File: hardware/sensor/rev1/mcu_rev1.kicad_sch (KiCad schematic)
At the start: 14 parts, among them IC1 STM8L051F3P6, J1 22-28-4044, J2 M20-9770342

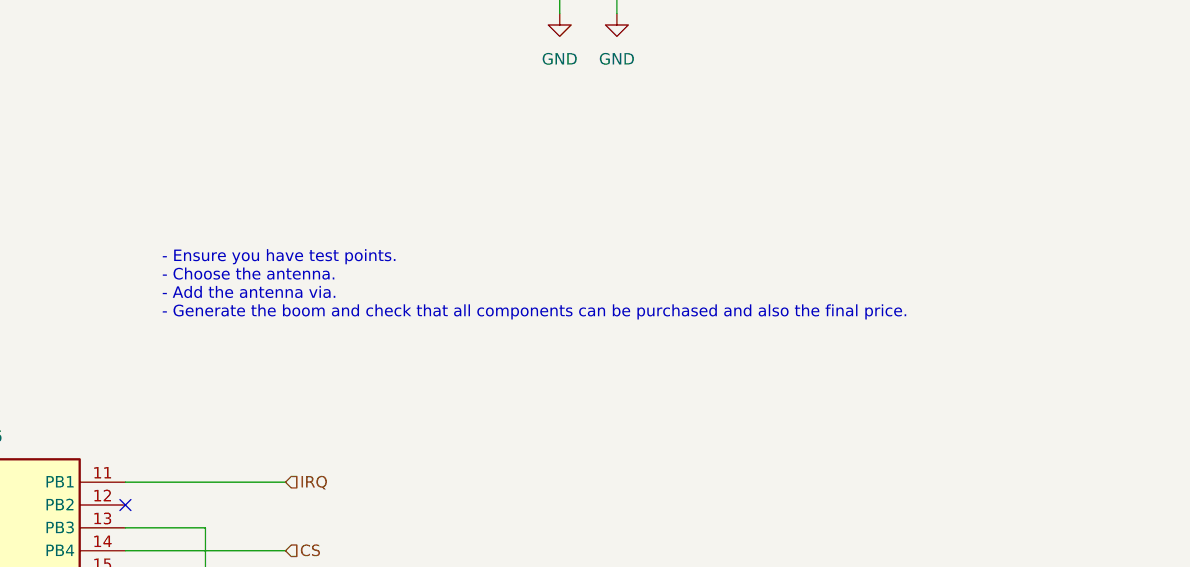
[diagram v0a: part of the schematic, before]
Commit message: EG-49 Adjust antenna place in PCB.
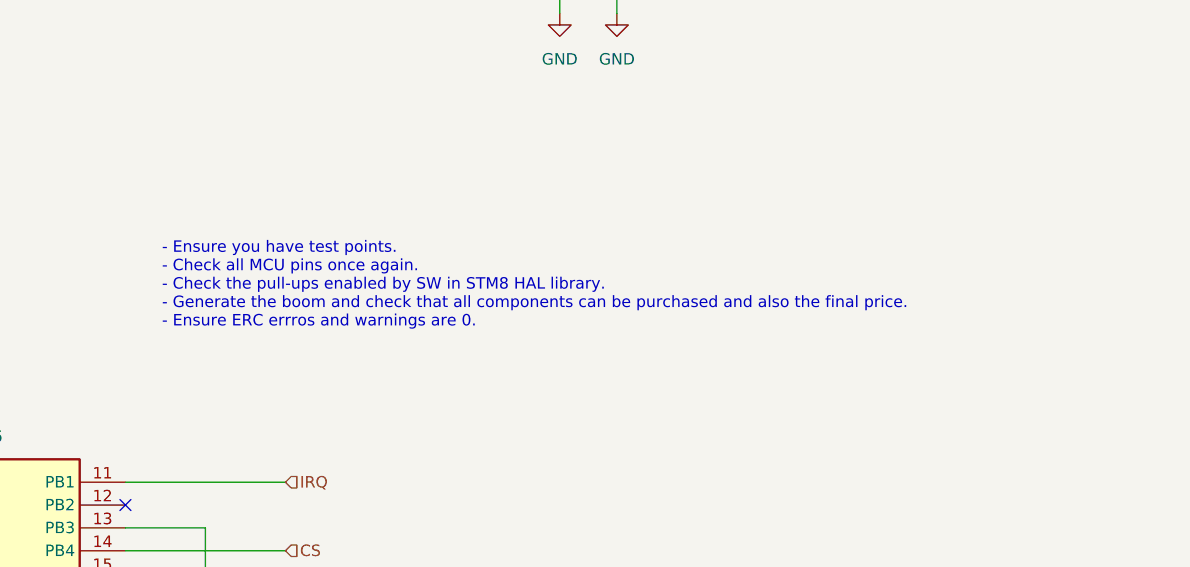
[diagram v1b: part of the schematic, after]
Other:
- note added: "- Ensure you have test points. - Check all MCU pins once again. - Check the pull-ups enabled by SW in STM8 HAL library. - Generate the boom and check that all components can be purchased and also the final price. - Ensure ERC errros and warnings are 0."
- note removed: "- Ensure you have test points. - Choose the antenna. - Add the antenna via. - Generate the boom and check that all components can be purchased and also the final price."
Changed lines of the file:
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@@
 		)
 	)
-	(text "- Ensure you have test points.\n- Choose the antenna.\n- Add the antenna via.\n- Generate the boom and check that all components can be purchased and also the final price."
+	(text "- Ensure you have test points.\n- Check all MCU pins once again.\n- Check the pull-ups enabled by SW in STM8 HAL library.\n- Generate the boom and check that all components can be purchased and also the final price.\n- Ensure ERC errros and warnings are 0."
 		(exclude_from_sim no)
 		(at 128.524 126.746 0)
